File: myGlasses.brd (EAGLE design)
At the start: 39.2 x 17.3 mm, 16 parts

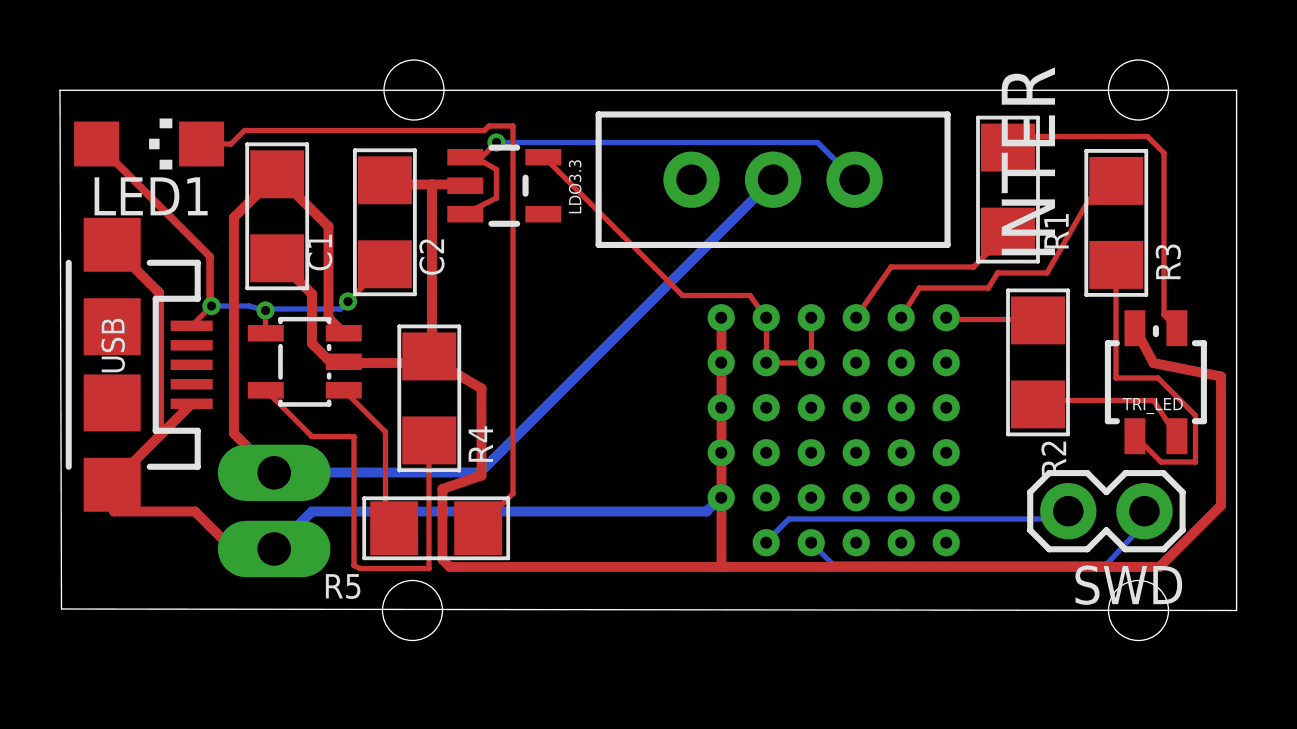
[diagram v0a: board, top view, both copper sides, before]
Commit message: Lunettes petit format corrige
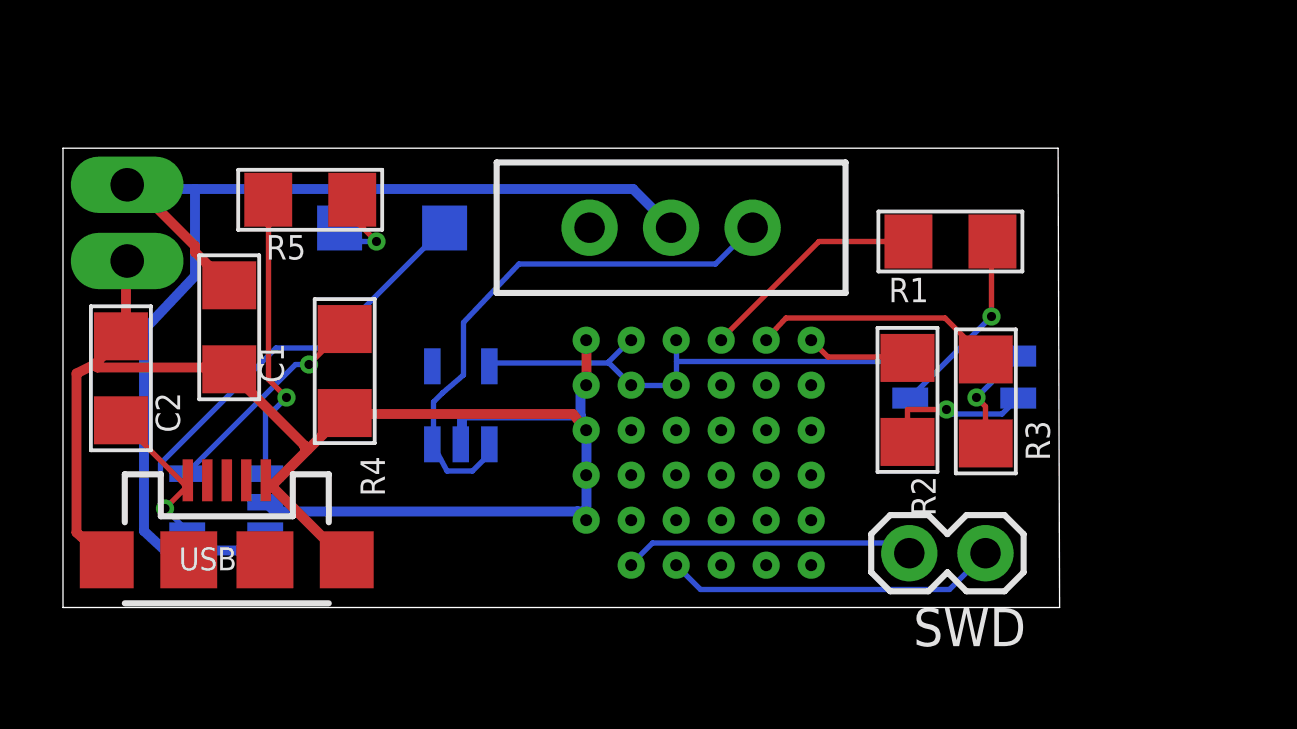
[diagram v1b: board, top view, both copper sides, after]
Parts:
- moved R5 11.7 mm to (8.29, 13.6)
- moved BATT 10.8 mm to (2.19, 11.6)
- moved C2 10.2 mm to (1.98, 7.69)
- moved LED1 8.57 mm to (11.0, 12.7), flipped to the bottom
- moved USB 7.54 mm to (5.51, 1.64), turned to 0 degrees
- moved LDO3.3 7.46 mm to (13.3, 6.79), flipped to the bottom, turned to 0 degrees
- moved R3 7.37 mm to (30.8, 6.92)
- moved TRI_LED 6.39 mm to (30.1, 7.73), flipped to the bottom, turned to 90 degrees
- moved SWD 5.48 mm to (30.8, 1.86)
- moved CHARG 5.36 mm to (5.49, 3.56), flipped to the bottom, turned to 270 degrees
- moved N550 4.56 mm to (25.0, 8.96)
- moved R2 4.53 mm to (28.2, 6.97)
- moved C1 4.03 mm to (5.59, 9.39)
- moved INTER 3.76 mm to (20.3, 12.7)
- moved R4 2.96 mm to (9.44, 7.93), turned to 270 degrees
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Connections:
- net 3.3V: now also TRI_LED.A
- net GND: no longer TRI_LED.A
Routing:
- net GND: track 101.8 -> 57.3 mm
- net N$9: track 24.5 -> 3.14 mm, vias 0 -> 1
- net N$7: track 14.9 -> 7.26 mm, vias 0 -> 1
- net N$4: track 10.9 -> 3.62 mm, vias 0 -> 1
- net N$2: track 11.8 -> 6.37 mm, vias 0 -> 1
- net N$5: track 15.1 -> 19.9 mm, vias 3 -> 1
- net N$8: track 5.31 -> 9.85 mm, vias 0 -> 1
- net 3.3V: track 14.2 -> 17.0 mm
- net N$1: track 38.2 -> 40.4 mm
- net VCC-ISO: track 17.0 -> 18.5 mm, vias 1 -> 0
- net N$12: track 9.62 -> 8.24 mm
- net N$10: track 12.4 -> 11.2 mm
- net N$11: track 6.46 -> 7.62 mm
- net N$6: track 10.5 -> 9.75 mm
- net N$3: track 5.40 -> 5.05 mm, vias 0 -> 1
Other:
- board size 39.2 x 17.3 mm -> 33.2 x 15.3 mm
